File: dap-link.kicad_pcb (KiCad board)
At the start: 4 copper layers, 65 x 30 mm, 46 parts, among them J1 Molex 0473460001, J2 Conn_01x05_Male, J3 SWD 10 pin 2.54mm, J4 SWD 10 pin 1.27mm, Q1 MMBT3904, U1 SC573V33RTRC, U2 STM32F103CBTx, U3 150141SV73110, Y1 8MHz

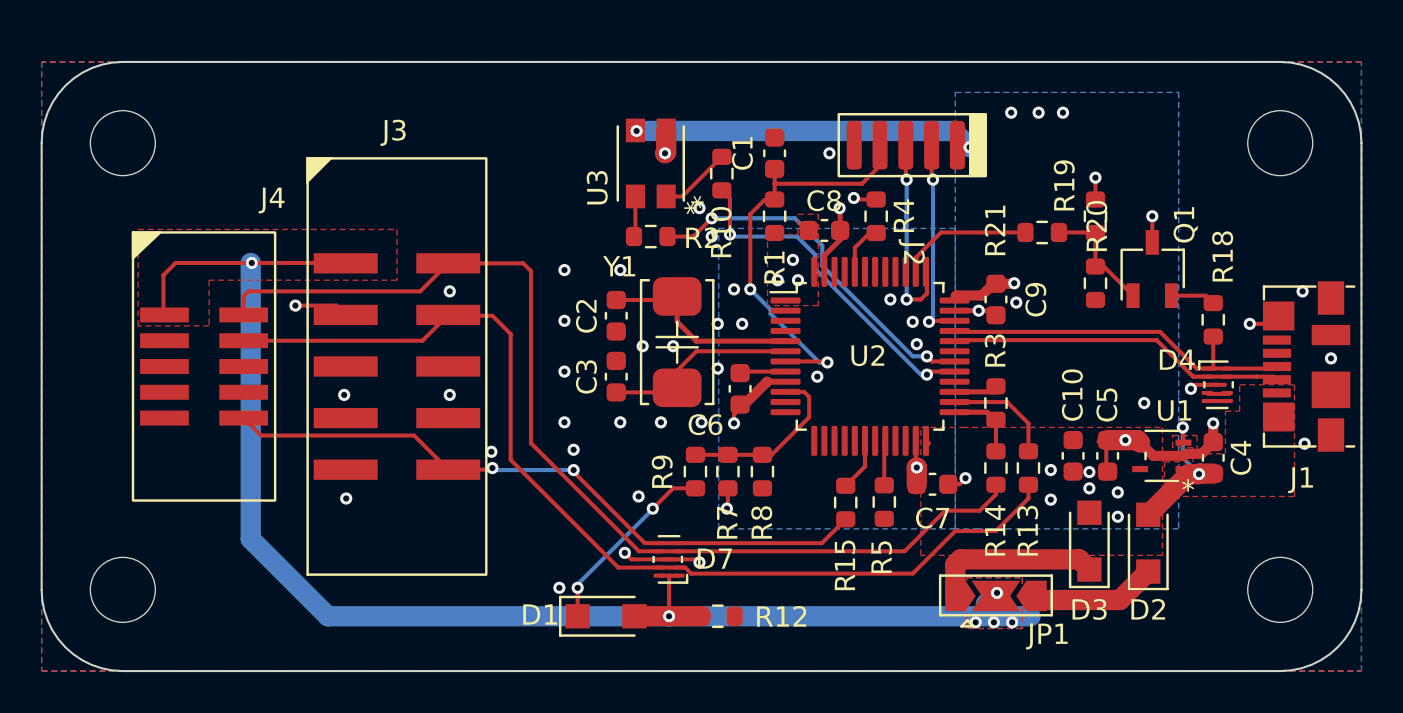
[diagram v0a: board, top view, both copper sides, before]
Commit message: changes
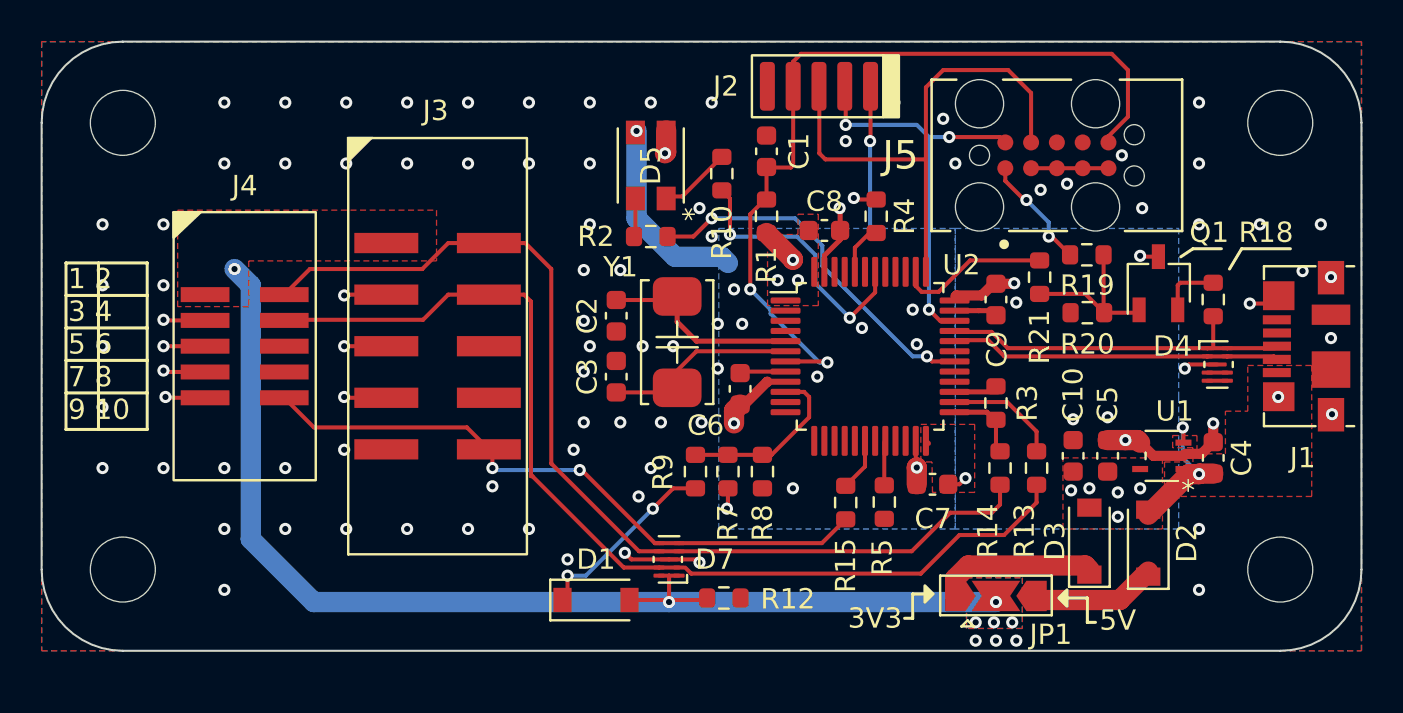
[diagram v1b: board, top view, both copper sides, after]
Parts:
- removed U3: 150141SV73110, MyLib:150141SV73110
- added D5: 150141SV73110, MyLib:150141SV73110, F.Cu at (73.0, 66.1)
- added J5: TC2050-IDC, MyLib:TAG-CONNECT_TC2050-IDC, F.Cu at (93.0, 65.6)
- C2, C3: value 20p -> 18p
- D1, D2, D3: value D_Small -> SM5817PL-TP; footprint Diode_SMD:Nexperia_CFP3_SOD-123W -> Diode_SMD:D_SOD-123
- moved J2 5.17 mm to (81.3, 62.2)
- moved J3 2.24 mm to (62.5, 75.0)
- moved J4 2.24 mm to (53.0, 75.0)
- moved R21 2.20 mm to (92.2, 71.6), turned to -90 degrees
- moved R19 1.95 mm to (94.5, 70.5), turned to 180 degrees
- moved R20 1.50 mm to (94.5, 73.3), turned to 0 degrees
- moved D4 1.00 mm to (100.9, 75.9)
- moved H1 1.00 mm to (104.0, 64.0)
- moved H2 1.00 mm to (104.0, 86.0)
- moved H3 1.00 mm to (47.0, 86.0)
- moved H4 1.00 mm to (47.0, 64.0)
- moved J1 1.00 mm to (106.5, 75.0)
- moved R18 1.00 mm to (100.7, 72.7)
- moved R12 0.95 mm to (76.6, 87.4)
- moved D1 0.94 mm to (70.3, 87.5)
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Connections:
- net Net-(D1-Pad1) renamed /T_VTREF
- U2 pad 29: /CONNECTED_LED -> unconnected-(U2-Pad29)
- U2 pad 42: unconnected-(U2-Pad42) -> /CONNECTED_LED
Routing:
- net STM_NRST: track 20.7 -> 41.2 mm
- net STM_SWCLK: track 10.1 -> 26.2 mm, vias 2 -> 0
- net VTREF: track 71.9 -> 57.9 mm
- net GND: track 30.9 -> 44.5 mm, vias 49 -> 105
- net STM_SWDIO: track 10.1 -> 20.1 mm, vias 2 -> 3
- net +3V3: track 30.0 -> 37.3 mm
- net /CONNECTED_LED: track 16.7 -> 13.5 mm
- net Net-(Q1-Pad1): track 5.87 -> 7.97 mm
- net SWCLK: track 49.7 -> 51.1 mm
- net NRST: track 32.8 -> 31.5 mm
- net SWDIO: track 51.2 -> 50.1 mm
- net /USB_RENUMn: track 6.61 -> 7.56 mm
- net Net-(Q1-Pad2): track 2.20 -> 3.01 mm
- net Net-(D3-Pad1): track 8.45 -> 7.81 mm
- net /USB_DP: track 18.2 -> 17.6 mm
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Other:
- board text added: "1 2 3 4 5 6 7 8 9 10"
- board text added: "10 PIN SWD OUT (J3, J4)"
- board text added: "3V3"
- board text added: "5V"
- board text added: "NAME SWDIO SWCLK NC NC NRST"
- board text added: "PINOUT J2 1 3V3 2 SWDIO 3 SWCLK 4 NRST 5 GND"
- board text added: "PINOUT J5 3V3 SWDIO GND SWCLK GND NC GND NC GND NRST"
- board text added: "SET JP1 ON FRONT SIDE TO FORCE VTREF TO 3.3V OR 5V"
- board text added: "USE J2 OR J5 TO FLASH BOOTLOADER"
- board text removed: "10 PIN CONNECTOR PINOUT"
- board text removed: "20 PIN CONNECTOR PINOUT"
- board text removed: "6 PIN SWD"
- board text removed: "GND"
- board text removed: "Jumpers not set -> VTREF = VDUT Pos 1 set -> VTREF = 3V3 Pos 2 set -> VTREF = 5V"
- board text removed: "NAME SWDIO/TMS SWCLK/TCLK SWO TDI NRST"
- board text removed: "NAME VTREF GND GND GND GND GND GND GND GND GND"
- board text removed: "NAME VTREF NC TDI SWDIO/TMS SWCLK/TCLK NC SWO NRST NC NC"
- board text removed: "NR 1 3 5 7 9 11 13 15 17 19"
- board text removed: "NR 2 4 6 8 10 12 14 16 18 20"
- board text removed: "NRST"
- board text removed: "SWCLK"
- board text removed: "SWDIO"
- board text removed: "SWO"
- board text removed: "VTREF"
